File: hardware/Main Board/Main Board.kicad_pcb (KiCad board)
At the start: 4 copper layers, 65 x 56 mm, 29 parts, among them J1 Motor Power, J2 DEC Motor, J3 RA Motor, J4 Conn_01x05_Female, P1 Conn_02x20_Odd_Even, Q1 2N3904, Q2 2N3904, Q3 2N3904, Q4 2N3904, Q5 2N3904, U1 ELEGOO, U2 ELEGOO

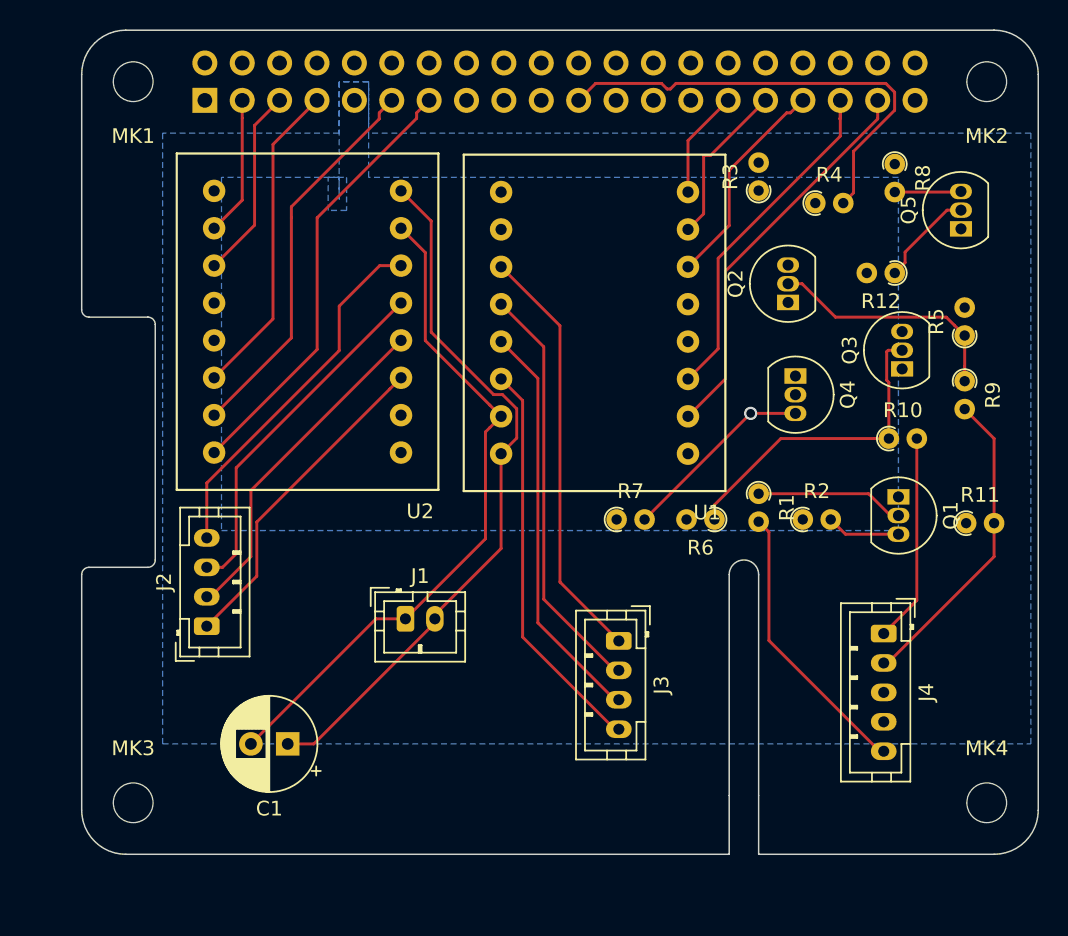
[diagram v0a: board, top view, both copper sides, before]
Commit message: First Routing...
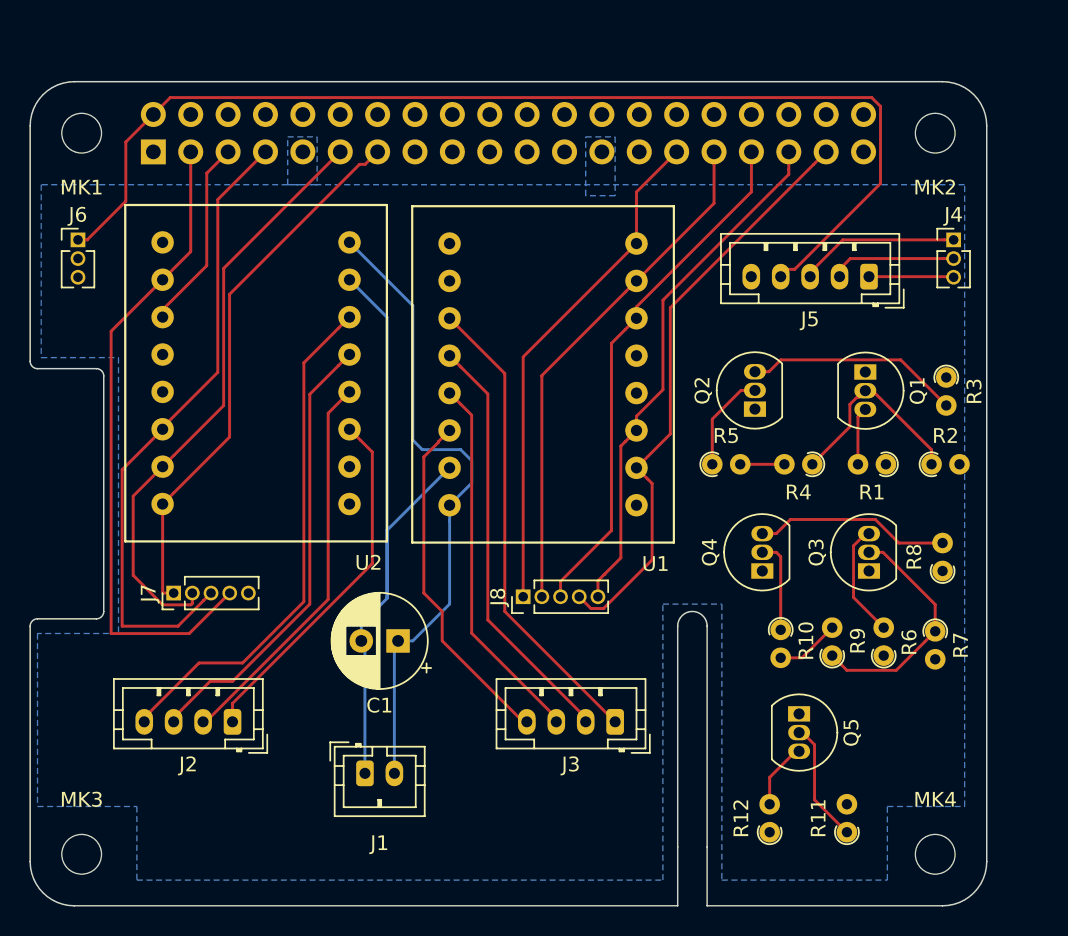
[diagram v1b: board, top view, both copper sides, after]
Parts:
- added J5: Joystick Connector, Connector_JST:JST_PH_B5B-PH-K_1x05_P2.00mm_Vertical, F.Cu at (253.5, 110.8)
- added J6: System Debug, Connector_PinHeader_1.27mm:PinHeader_1x03_P1.27mm_Vertical, F.Cu at (199.8, 108.2)
- added J7: DEC Debug, Connector_PinHeader_1.27mm:PinHeader_1x05_P1.27mm_Vertical, F.Cu at (206.2, 132.2)
- added J8: RA Debug, Connector_PinHeader_1.27mm:PinHeader_1x05_P1.27mm_Vertical, F.Cu at (230.0, 132.5)
- J4: value Conn_01x05_Female -> Joystick Debug; footprint Connector_JST:JST_PH_B5B-PH-K_1x05_P2.00mm_Vertical -> Connector_PinHeader_1.27mm:PinHeader_1x03_P1.27mm_Vertical
- R2, R7: value 100K -> 22K
- R5, R6: value 22K -> 100K
- U1: value ELEGOO -> RA Driver
- moved R12 38.9 mm to (246.8, 148.5), turned to 90 degrees
- moved Q5 34.7 mm to (248.8, 140.5), turned to 270 degrees
- moved R8 27.8 mm to (258.5, 130.8), turned to 90 degrees
- moved J4 27.2 mm to (259.2, 108.2), turned to 0 degrees
- moved R7 22.9 mm to (258.0, 134.8), turned to 270 degrees
- moved R11 22.5 mm to (252.0, 148.5), turned to 90 degrees
- moved R9 20.7 mm to (251.0, 136.5), turned to 90 degrees
- moved R5 19.3 mm to (242.8, 123.5), turned to 0 degrees
- moved R3 18.0 mm to (258.8, 117.6), turned to 270 degrees
- moved R4 17.8 mm to (249.7, 123.5), turned to 180 degrees
- moved R10 14.9 mm to (247.5, 134.8), turned to 270 degrees
- moved R6 14.8 mm to (254.5, 136.5), turned to 90 degrees
- moved Q3 13.9 mm to (253.5, 130.8)
- moved Q4 13.4 mm to (246.2, 130.8), turned to 90 degrees
- moved J1 10.9 mm to (219.2, 144.5)
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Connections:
- J4 pad 3: +5V -> Net-(J4-Pad3)
- P1 pad 25: Net-(P1-Pad25) -> GND
- Q1 pad 3: /GPIO10(SPI0_MOSI) -> /ID_SD
- Q2 pad 3: /ID_SD -> /GPIO22(GEN3)
- Q3 pad 3: /GPIO9(SPI0_MISO) -> /GPIO11(SPI0_SCK)
- Q4 pad 3: /GPIO25(GEN6) -> /GPIO9(SPI0_MISO)
- Q5 pad 3: /GPIO11(SPI0_SCK) -> /GPIO10(SPI0_MOSI)
- R1 pad 1: Net-(Q1-Pad2) -> +3V3
- R1 pad 2: Net-(J4-Pad5) -> /ID_SD
- R10 pad 1: Net-(Q3-Pad2) -> Net-(Q4-Pad2)
- R10 pad 2: Net-(J4-Pad1) -> Net-(J4-Pad3)
- R11 pad 1: Net-(Q4-Pad2) -> Net-(Q5-Pad2)
- R11 pad 2: Net-(J4-Pad2) -> Net-(J4-Pad1)
- R12 pad 1: Net-(Q5-Pad2) -> +3V3
- R12 pad 2: Net-(J4-Pad1) -> /GPIO10(SPI0_MOSI)
- R2 pad 1: +3V3 -> Net-(Q1-Pad2)
- R2 pad 2: /GPIO10(SPI0_MOSI) -> GND
- R3 pad 2: /ID_SD -> /GPIO22(GEN3)
- R4 pad 1: +3V3 -> Net-(Q1-Pad2)
- R4 pad 2: /GPIO9(SPI0_MISO) -> Net-(J4-Pad2)
- R5 pad 2: GND -> Net-(J4-Pad2)
- R6 pad 1: Net-(Q3-Pad2) -> +3V3
- R6 pad 2: GND -> /GPIO11(SPI0_SCK)
- R7 pad 1: +3V3 -> Net-(Q3-Pad2)
- R7 pad 2: /GPIO25(GEN6) -> GND
- R8 pad 2: /GPIO11(SPI0_SCK) -> /GPIO9(SPI0_MISO)
- R9 pad 1: Net-(Q2-Pad2) -> Net-(Q3-Pad2)
- R9 pad 2: Net-(J4-Pad2) -> Net-(J4-Pad3)
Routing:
- net /GPIO22(GEN3): track 0.00 -> 48.7 mm
- net /GPIO25(GEN6): track 43.0 -> 0.00 mm, vias 1 -> 0
- net Net-(J4-Pad3): track 0.00 -> 37.4 mm
- net /GPIO2(SDA1): track 9.48 -> 44.2 mm
- net Net-(J4-Pad1): track 28.1 -> 56.3 mm
- net /GPIO5: track 7.36 -> 34.5 mm
- net +3V3: track 0.00 -> 24.4 mm
- net /GPIO6: track 11.2 -> 35.1 mm
- net /GPIO4(GCLK): track 21.7 -> 43.2 mm
- net /GPIO3(SCL1): track 13.1 -> 34.5 mm
- net /GPIO13(PWM1): track 14.7 -> 35.6 mm
- net Net-(J4-Pad5): track 19.3 -> 0.00 mm
- net /GPIO11(SPI0_SCK): track 27.5 -> 43.9 mm
- net /ID_SD: track 14.2 -> 28.4 mm
- net /GPIO17(GEN0): track 26.4 -> 40.2 mm
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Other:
- net class Motor Power added: clearance 0.2, trace_width 0.2, via_dia 0.9, via_drill 0.6
- board text removed: "RASPBERRY-PI 40-PIN ADDON BOARD VIEW FROM TOP NOTE: P1 SHOULD BE FITTED ON THE REVERSE OF THE BOARD ADD EDGE CUTS FROM CAMERA AND DISPLAY PORTS AS REQUIRED"
- board text removed: "RJ45"
- board text removed: "USB"

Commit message: Ready to Build the Board
release_1.0
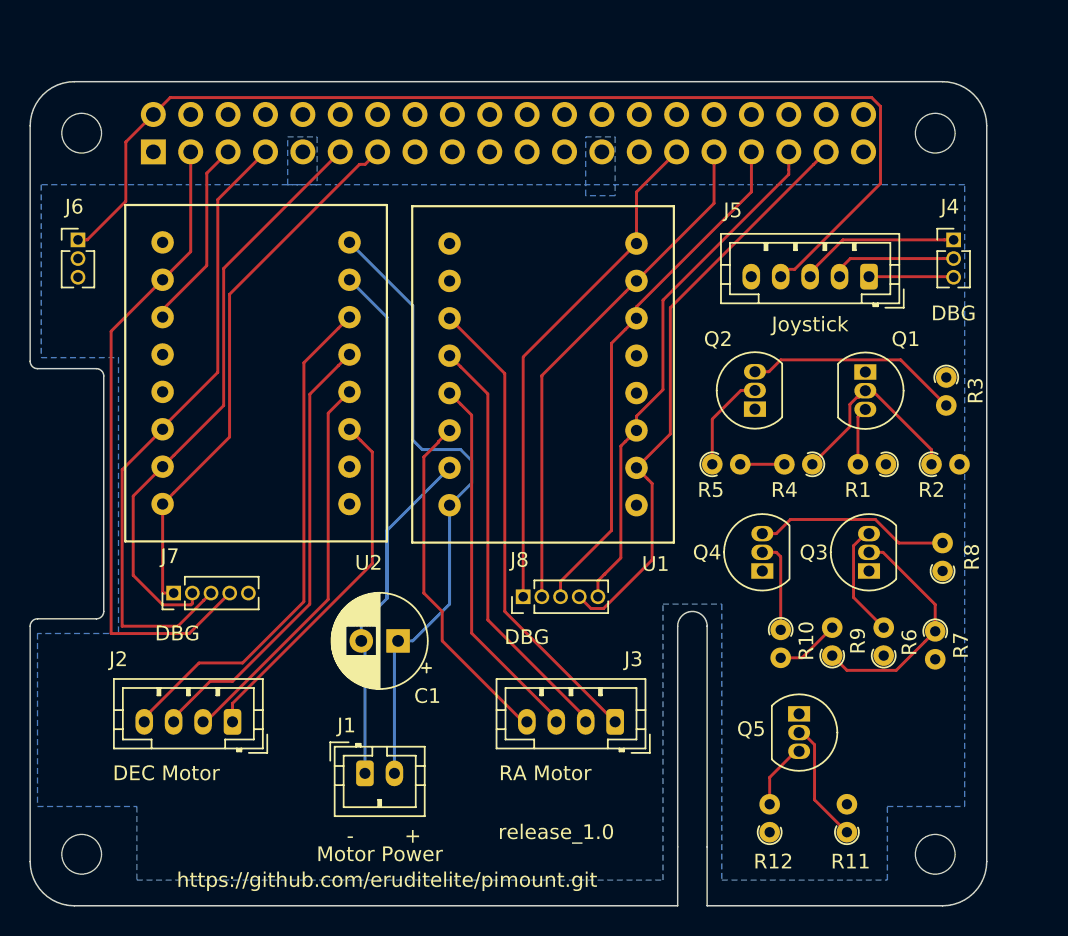
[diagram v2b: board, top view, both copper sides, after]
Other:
- board text added: "+"
- board text added: "-"
- board text added: "DBG"
- board text added: "DEC Motor"
- board text added: "Joystick"
- board text added: "Motor Power"
- board text added: "RA Motor"
- board text added: "https://github.com/eruditelite/pimount.git"
- board text added: "release_1.0"
